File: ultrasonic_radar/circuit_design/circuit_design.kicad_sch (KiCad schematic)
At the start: 11 parts

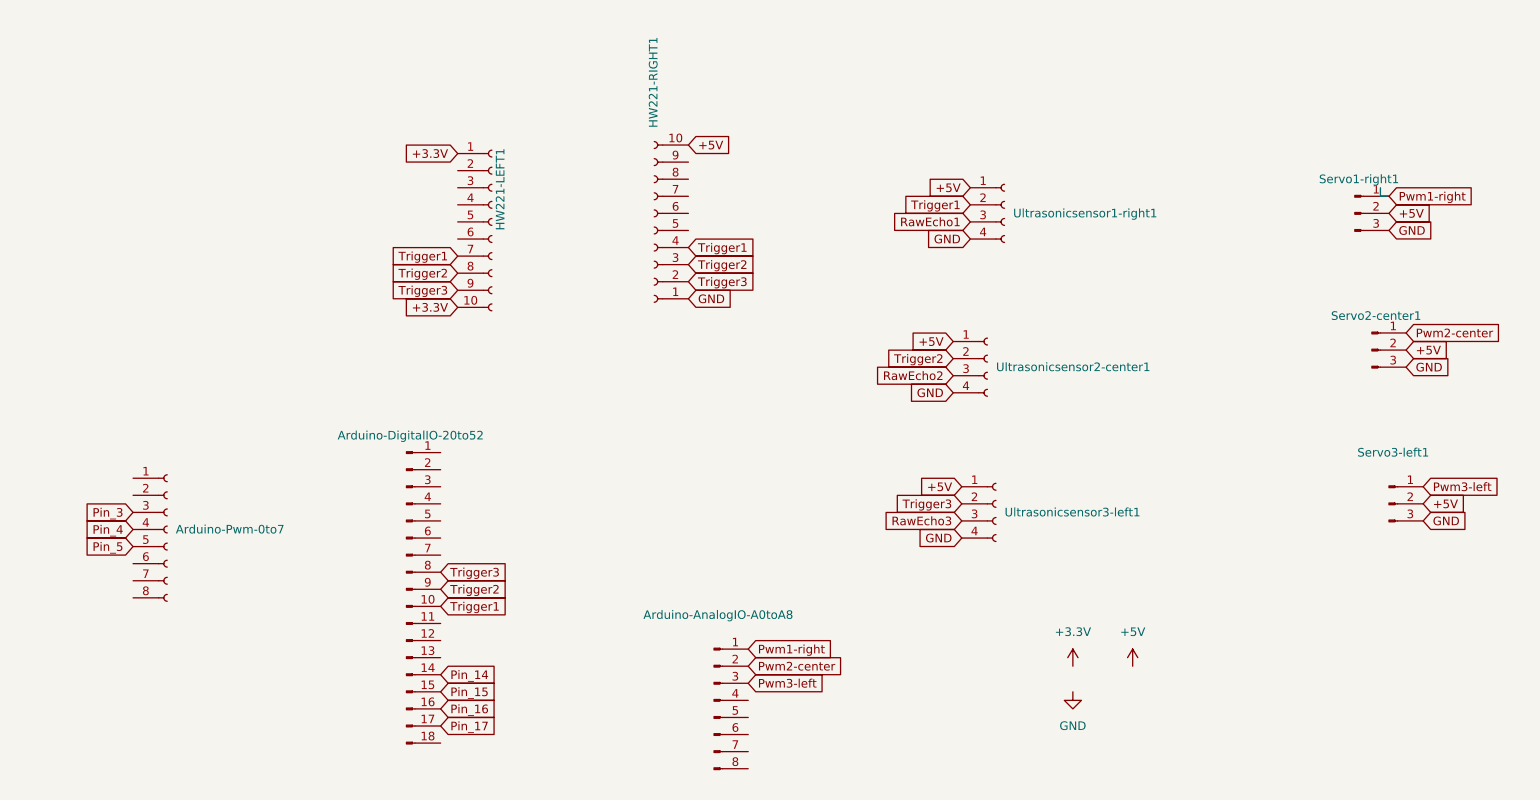
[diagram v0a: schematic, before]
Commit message: circuit pcb design updated
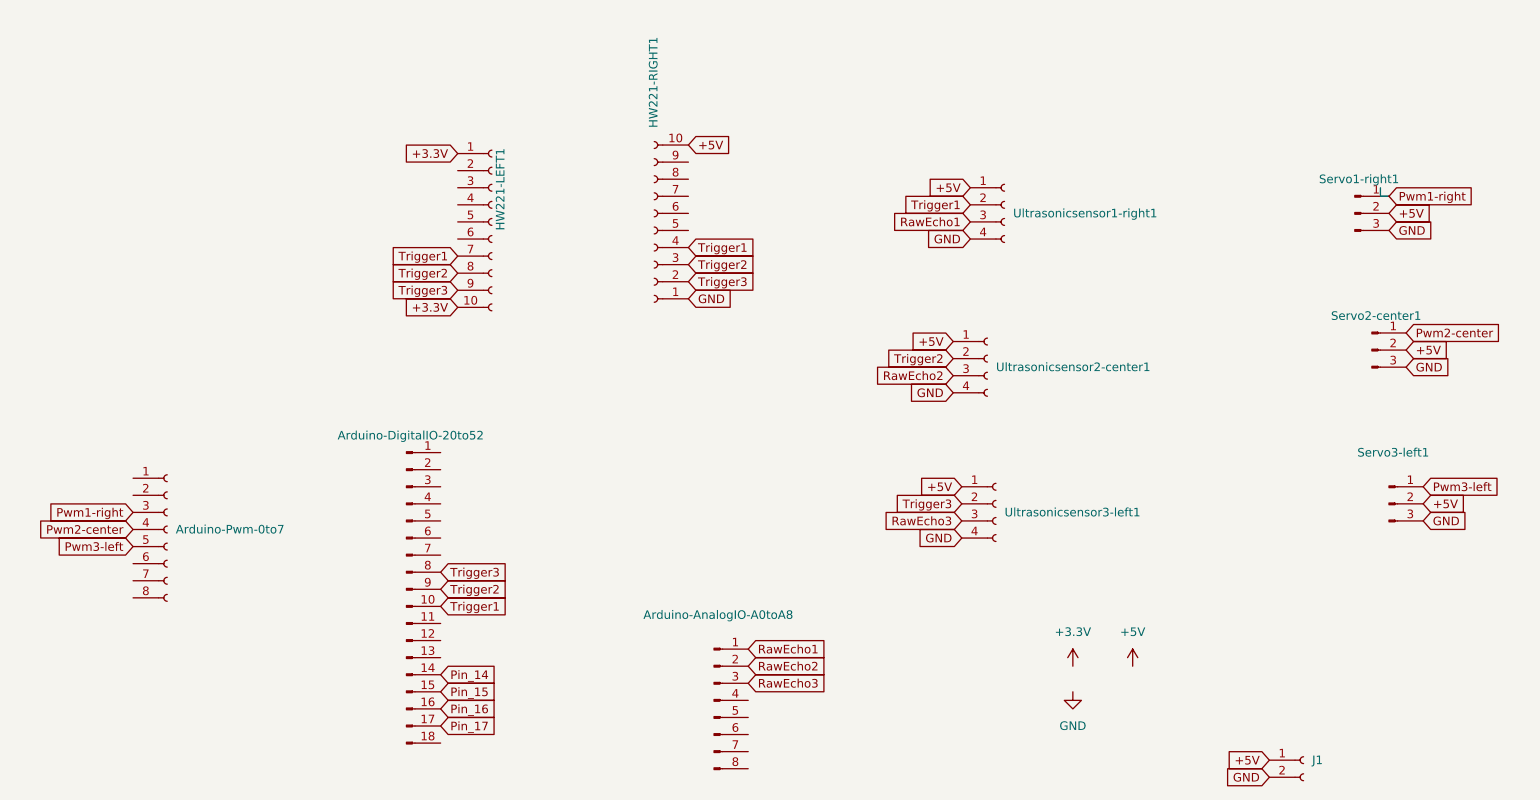
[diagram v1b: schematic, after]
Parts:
- added J1: Conn_01x02_Socket, Connector_Molex:Molex_KK-396_5273-02A_1x02_P3.96mm_Vertical, symbol Connector:Conn_01x02_Socket
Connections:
- net Pin_3 is gone; now on net Pwm1-right: Arduino-Pwm-0to7.3 (Pin_3)
- net Pin_4 is gone; now on net Pwm2-center: Arduino-Pwm-0to7.4 (Pin_4)
- net Pin_5 is gone; now on net Pwm3-left: Arduino-Pwm-0to7.5 (Pin_5)
- net +5V: now also J1.1 (Pin_1)
- net GND: now also J1.2 (Pin_2)
- net Pwm1-right: no longer Arduino-AnalogIO-A0toA8.1 (Pin_1)
- net Pwm2-center: no longer Arduino-AnalogIO-A0toA8.2 (Pin_2)
- net Pwm3-left: no longer Arduino-AnalogIO-A0toA8.3 (Pin_3)
- net RawEcho1: now also Arduino-AnalogIO-A0toA8.1 (Pin_1)
- net RawEcho2: now also Arduino-AnalogIO-A0toA8.2 (Pin_2)
- net RawEcho3: now also Arduino-AnalogIO-A0toA8.3 (Pin_3)
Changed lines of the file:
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@@
 		)
 	)
-	(global_label "Pin_3"
+	(global_label "Pwm1-right"
 		(shape input)
 		(at 29.21 113.03 180)
@@
 	(global_label "GND"
 		(shape input)
+		(at 198.12 152.4 180)
+		(effects
+			(font
+				(size 1.27 1.27)
+			)
+			(justify right)
+		)
+		(property "Intersheetrefs" "${INTERSHEET_REFS}"
+			(at 198.12 152.4 0)
+			(effects
+				(font
+					(size 1.27 1.27)
+				)
+				(hide yes)
+			)
+		)
+	)
+	(global_label "GND"
+		(shape input)
 		(at 111.76 81.28 0)
 		(effects
@@
 		)
 	)
+	(global_label "RawEcho3"
+		(shape input)
+		(at 120.65 138.43 0)
+		(effects
+			(font
+				(size 1.27 1.27)
+			)
+			(justify left)
+		)
+		(property "Intersheetrefs" "${INTERSHEET_REFS}"
+			(at 120.65 138.43 0)
+			(effects
+				(font
+					(size 1.27 1.27)
+				)
+				(hide yes)
+			)
+		)
+	)
 	(global_label "Pwm3-left"
 		(shape input)
-		(at 120.65 138.43 0)
-		(effects
-			(font
-				(size 1.27 1.27)
-			)
-			(justify left)
-		)
-		(property "Intersheetrefs" "${INTERSHEET_REFS}"
-			(at 120.65 138.43 0)
-			(effects
-				(font
-					(size 1.27 1.27)
-				)
-				(hide yes)
-			)
-		)
-	)
-	(global_label "Pin_5"
-		(shape input)
 		(at 29.21 118.11 180)
 		(effects
@@
 		)
 	)
+	(global_label "RawEcho2"
+		(shape input)
+		(at 120.65 135.89 0)
+		(effects
+			(font
+				(size 1.27 1.27)
+			)
+			(justify left)
+		)
+		(property "Intersheetrefs" "${INTERSHEET_REFS}"
+			(at 120.65 135.89 0)
+			(effects
+				(font
+					(size 1.27 1.27)
+				)
+				(hide yes)
+			)
+		)
+	)
+	(global_label "Pwm1-right"
+		(shape input)
+		(at 215.9 66.04 0)
+		(effects
+			(font
+				(size 1.27 1.27)
+			)
+			(justify left)
+		)
+		(property "Intersheetrefs" "${INTERSHEET_REFS}"
+			(at 215.9 66.04 0)
+			(effects
+				(font
+					(size 1.27 1.27)
+				)
+				(hide yes)
+			)
+		)
+	)
+	(global_label "Pin_17"
+		(shape input)
+		(at 74.93 144.78 0)
+		(effects
+			(font
+				(size 1.27 1.27)
+			)
+			(justify left)
+		)
+		(property "Intersheetrefs" "${INTERSHEET_REFS}"
+			(at 74.93 144.78 0)
+			(effects
+				(font
+					(size 1.27 1.27)
+				)
+				(hide yes)
+			)
+		)
+	)
+	(global_label "Trigger1"
+		(shape input)
+		(at 74.93 127 0)
+		(effects
+			(font
+				(size 1.27 1.27)
+			)
+			(justify left)
+		)
+		(property "Intersheetrefs" "${INTERSHEET_REFS}"
+			(at 74.93 127 0)
+			(effects
+				(font
+					(size 1.27 1.27)
+				)
+				(hide yes)
+			)
+		)
+	)
+	(global_label "RawEcho1"
+		(shape input)
+		(at 120.65 133.35 0)
+		(effects
+			(font
+				(size 1.27 1.27)
+			)
+			(justify left)
+		)
+		(property "Intersheetrefs" "${INTERSHEET_REFS}"
+			(at 120.65 133.35 0)
+			(effects
+				(font
+					(size 1.27 1.27)
+				)
+				(hide yes)
+			)
+		)
+	)
+	(global_label "GND"
+		(shape input)
+		(at 151.13 95.25 180)
+		(effects
+			(font
+				(size 1.27 1.27)
+			)
+			(justify right)
+		)
+		(property "Intersheetrefs" "${INTERSHEET_REFS}"
+			(at 151.13 95.25 0)
+			(effects
+				(font
+					(size 1.27 1.27)
+				)
+				(hide yes)
+			)
+		)
+	)
 	(global_label "Pwm2-center"
 		(shape input)
-		(at 120.65 135.89 0)
-		(effects
-			(font
-				(size 1.27 1.27)
-			)
-			(justify left)
-		)
-		(property "Intersheetrefs" "${INTERSHEET_REFS}"
-			(at 120.65 135.89 0)
-			(effects
-				(font
-					(size 1.27 1.27)
-				)
-				(hide yes)
-			)
-		)
-	)
-	(global_label "Pwm1-right"
-		(shape input)
-		(at 215.9 66.04 0)
-		(effects
-			(font
-				(size 1.27 1.27)
-			)
-			(justify left)
-		)
-		(property "Intersheetrefs" "${INTERSHEET_REFS}"
-			(at 215.9 66.04 0)
-			(effects
-				(font
-					(size 1.27 1.27)
-				)
-				(hide yes)
-			)
-		)
-	)
-	(global_label "Pin_17"
-		(shape input)
-		(at 74.93 144.78 0)
-		(effects
-			(font
-				(size 1.27 1.27)
-			)
-			(justify left)
-		)
-		(property "Intersheetrefs" "${INTERSHEET_REFS}"
-			(at 74.93 144.78 0)
+		(at 29.21 115.57 180)
+		(effects
+			(font
+				(size 1.27 1.27)
+			)
+			(justify right)
+		)
+		(property "Intersheetrefs" "${INTERSHEET_REFS}"
+			(at 29.21 115.57 0)
 			(effects
 				(font
@@
 	(global_label "Trigger1"
 		(shape input)
-		(at 74.93 127 0)
-		(effects
-			(font
-				(size 1.27 1.27)
-			)
-			(justify left)
-		)
-		(property "Intersheetrefs" "${INTERSHEET_REFS}"
-			(at 74.93 127 0)
-			(effects
-				(font
-					(size 1.27 1.27)
-				)
-				(hide yes)
-			)
-		)
-	)
-	(global_label "Pwm1-right"
-		(shape input)
-		(at 120.65 133.35 0)
-		(effects
-			(font
-				(size 1.27 1.27)
-			)
-			(justify left)
-		)
-		(property "Intersheetrefs" "${INTERSHEET_REFS}"
-			(at 120.65 133.35 0)
+		(at 111.76 73.66 0)
+		(effects
+			(font
+				(size 1.27 1.27)
+			)
+			(justify left)
+		)
+		(property "Intersheetrefs" "${INTERSHEET_REFS}"
+			(at 111.76 73.66 0)
 			(effects
 				(font
@@
 	(global_label "GND"
 		(shape input)
-		(at 151.13 95.25 180)
-		(effects
-			(font
-				(size 1.27 1.27)
-			)
-			(justify right)
-		)
-		(property "Intersheetrefs" "${INTERSHEET_REFS}"
-			(at 151.13 95.25 0)
-			(effects
-				(font
-					(size 1.27 1.27)
-				)
-				(hide yes)
-			)
-		)
-	)
-	(global_label "Pin_4"
-		(shape input)
-		(at 29.21 115.57 180)
-		(effects
-			(font
-				(size 1.27 1.27)
-			)
-			(justify right)
-		)
-		(property "Intersheetrefs" "${INTERSHEET_REFS}"
-			(at 29.21 115.57 0)
-			(effects
-				(font
-					(size 1.27 1.27)
-				)
-				(hide yes)
-			)
-		)
-	)
-	(global_label "Trigger1"
-		(shape input)
-		(at 111.76 73.66 0)
-		(effects
-			(font
-				(size 1.27 1.27)
-			)
-			(justify left)
-		)
-		(property "Intersheetrefs" "${INTERSHEET_REFS}"
-			(at 111.76 73.66 0)
-			(effects
-				(font
-					(size 1.27 1.27)
-				)
-				(hide yes)
-			)
-		)
-	)
-	(global_label "GND"
-		(shape input)
 		(at 153.67 72.39 180)
 		(effects
@@
 		(property "Intersheetrefs" "${INTERSHEET_REFS}"
 			(at 77.47 59.69 0)
+			(effects
+				(font
+					(size 1.27 1.27)
+				)
+				(hide yes)
+			)
+		)
+	)
+	(global_label "+5V"
+		(shape input)
+		(at 198.12 149.86 180)
+		(effects
+			(font
+				(size 1.27 1.27)
+			)
+			(justify right)
+		)
+		(property "Intersheetrefs" "${INTERSHEET_REFS}"
+			(at 198.12 149.86 0)
 			(effects
 				(font
@@
 					(unit 1)
 				)
+			)
+		)
+	)
+	(symbol
+		(lib_id "Connector:Conn_01x02_Socket")
+		(at 203.2 149.86 0)
+		(unit 1)
+		(exclude_from_sim no)
+		(in_bom yes)
+		(on_board yes)
+		(dnp no)
+		(fields_autoplaced yes)
+		(property "Reference" "J1"
+			(at 204.47 149.8599 0)
+			(effects
+				(font
+					(size 1.27 1.27)
+				)
+				(justify left)
+			)
+		)
+		(property "Value" "Conn_01x02_Socket"
+			(at 204.47 152.3999 0)
+			(effects
+				(font
+					(size 1.27 1.27)
+				)
+				(justify left)
+				(hide yes)
+			)
+		)
+		(property "Footprint" "Connector_Molex:Molex_KK-396_5273-02A_1x02_P3.96mm_Vertical"
+			(at 203.2 149.86 0)
+			(effects
+				(font
+					(size 1.27 1.27)
+				)
+				(hide yes)
+			)
+		)
+		(property "Datasheet" "~"
+			(at 203.2 149.86 0)
+			(effects
+				(font
+					(size 1.27 1.27)
+				)
+				(hide yes)
+			)
+		)
+		(property "Description" "Generic connector, single row, 01x02, script generated"
+			(at 203.2 149.86 0)
+			(effects
+				(font
+					(size 1.27 1.27)
+				)
+				(hide yes)
+			)
+		)
+		(pin "1"
+		)
+		(pin "2"
+		)
+		(instances
+			(project ""
+				(path "/b8416165-cca2-412a-926f-d15dbbcb1a03"
+					(reference "J1")
+					(unit 1)
+				)
